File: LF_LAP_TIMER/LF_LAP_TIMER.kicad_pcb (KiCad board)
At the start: 2 copper layers, 94.5 x 64.5 mm, 21 parts, among them J1 SENSOR TERMINAL, J2 SENSOR TERMINAL, J3 LCD TERMINAL, SW1 ARM, SW2 STOP, SW3 RESTART

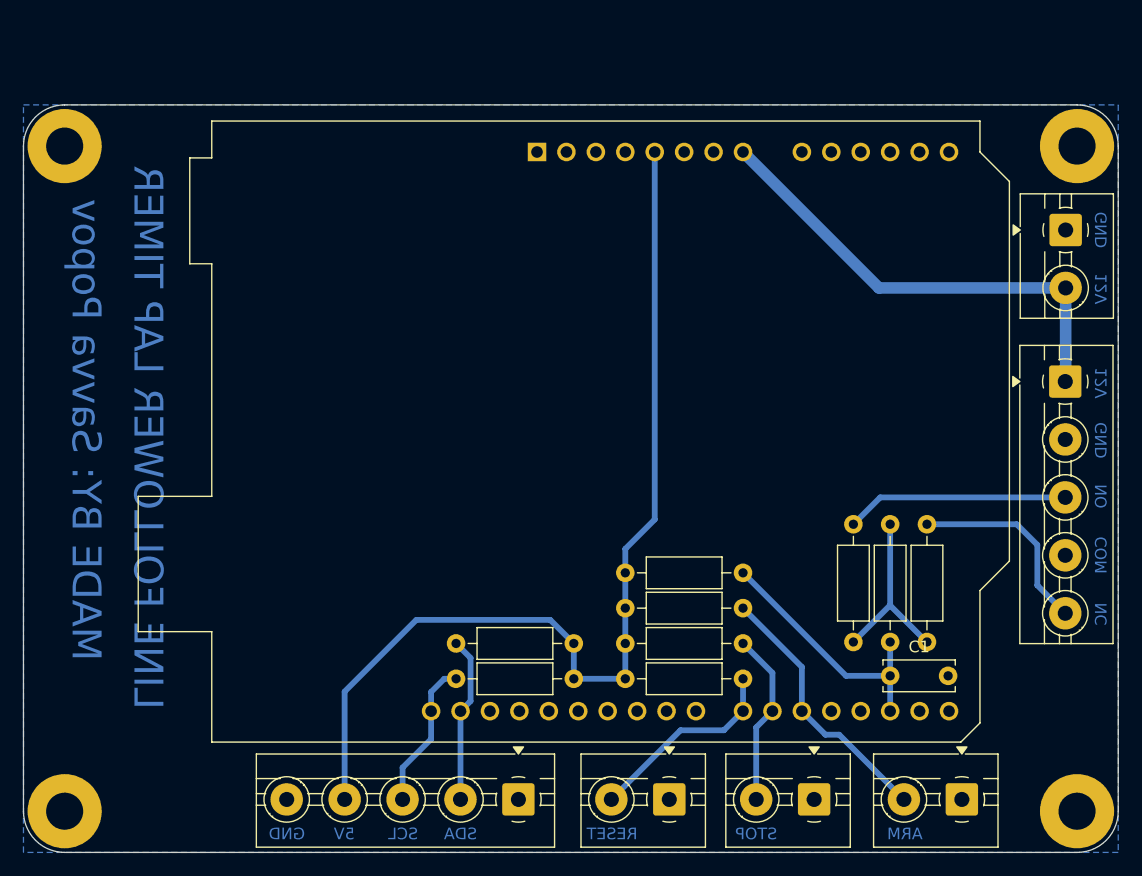
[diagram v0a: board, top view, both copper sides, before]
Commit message: Lap timer plots
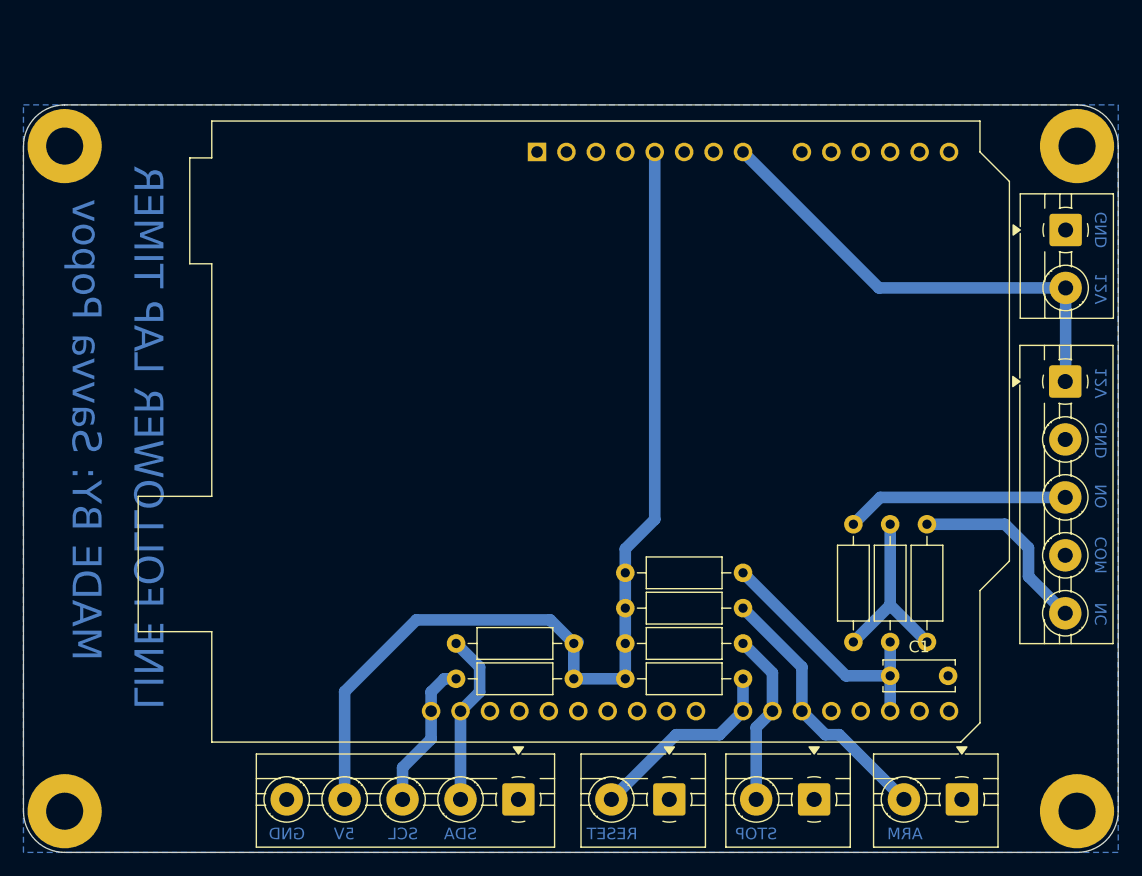
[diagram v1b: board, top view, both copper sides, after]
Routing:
- net SDA: track 14.5 -> 15.1 mm
- net RELAY_OUT_NC: track 17.2 -> 16.6 mm
